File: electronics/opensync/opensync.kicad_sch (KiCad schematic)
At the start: 0 parts

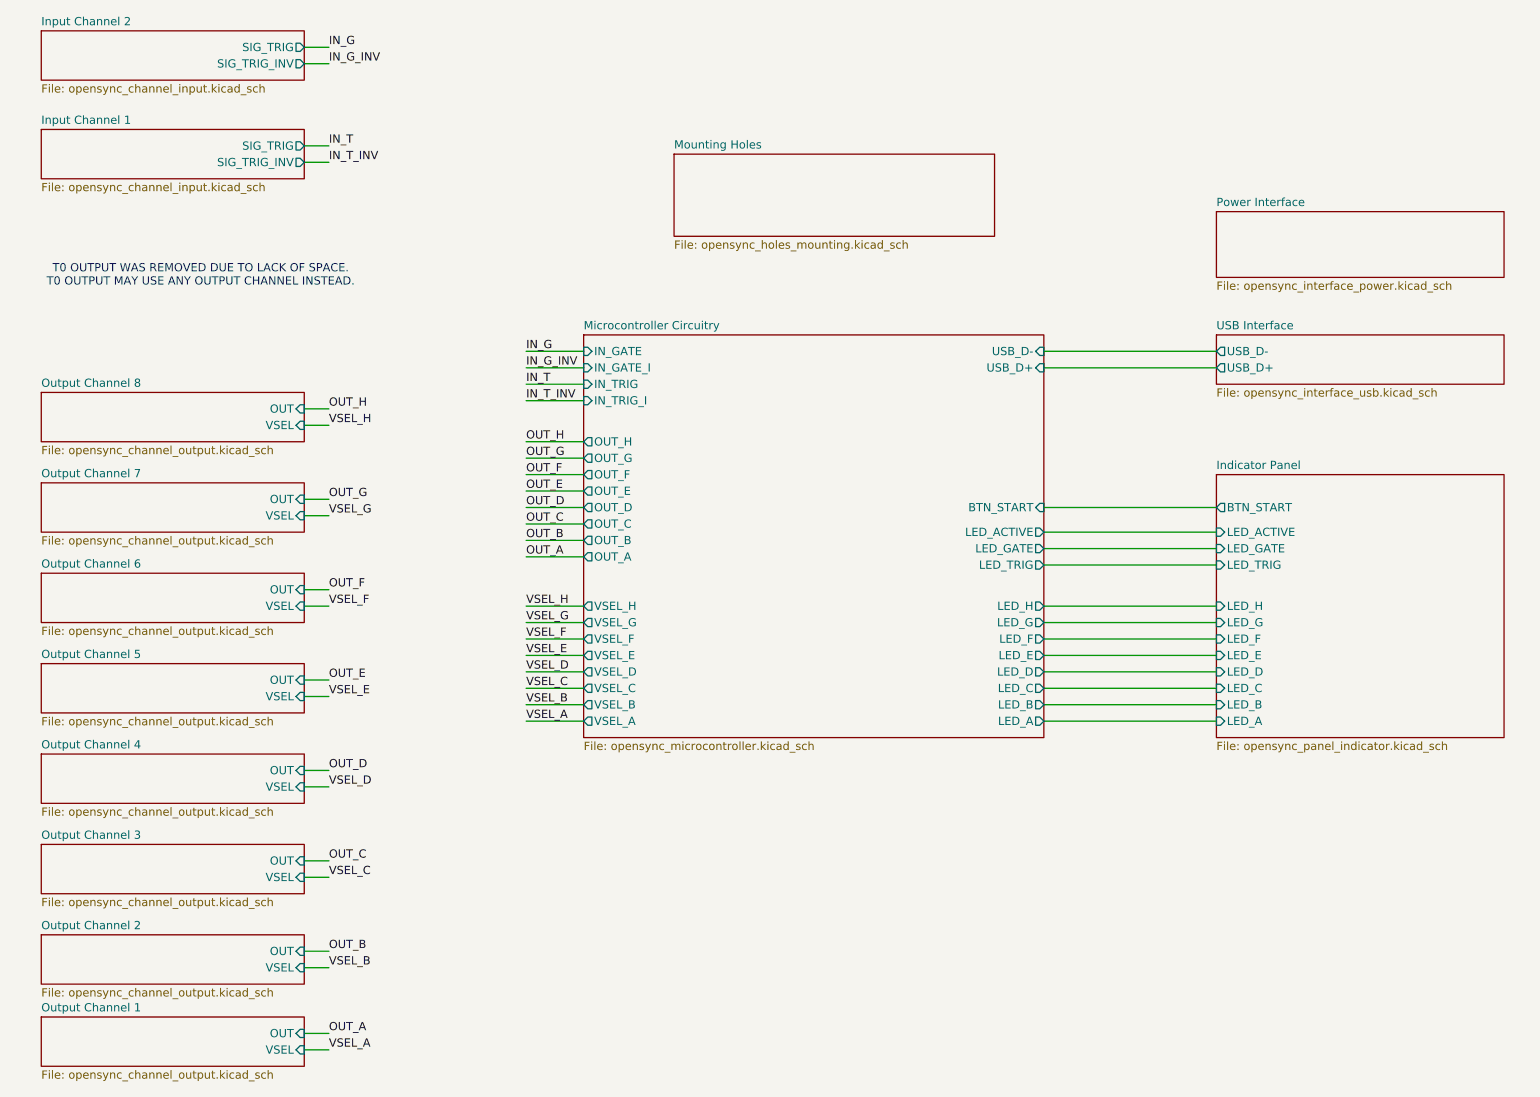
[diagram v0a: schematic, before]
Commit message: Updated new design; getting new PCBs
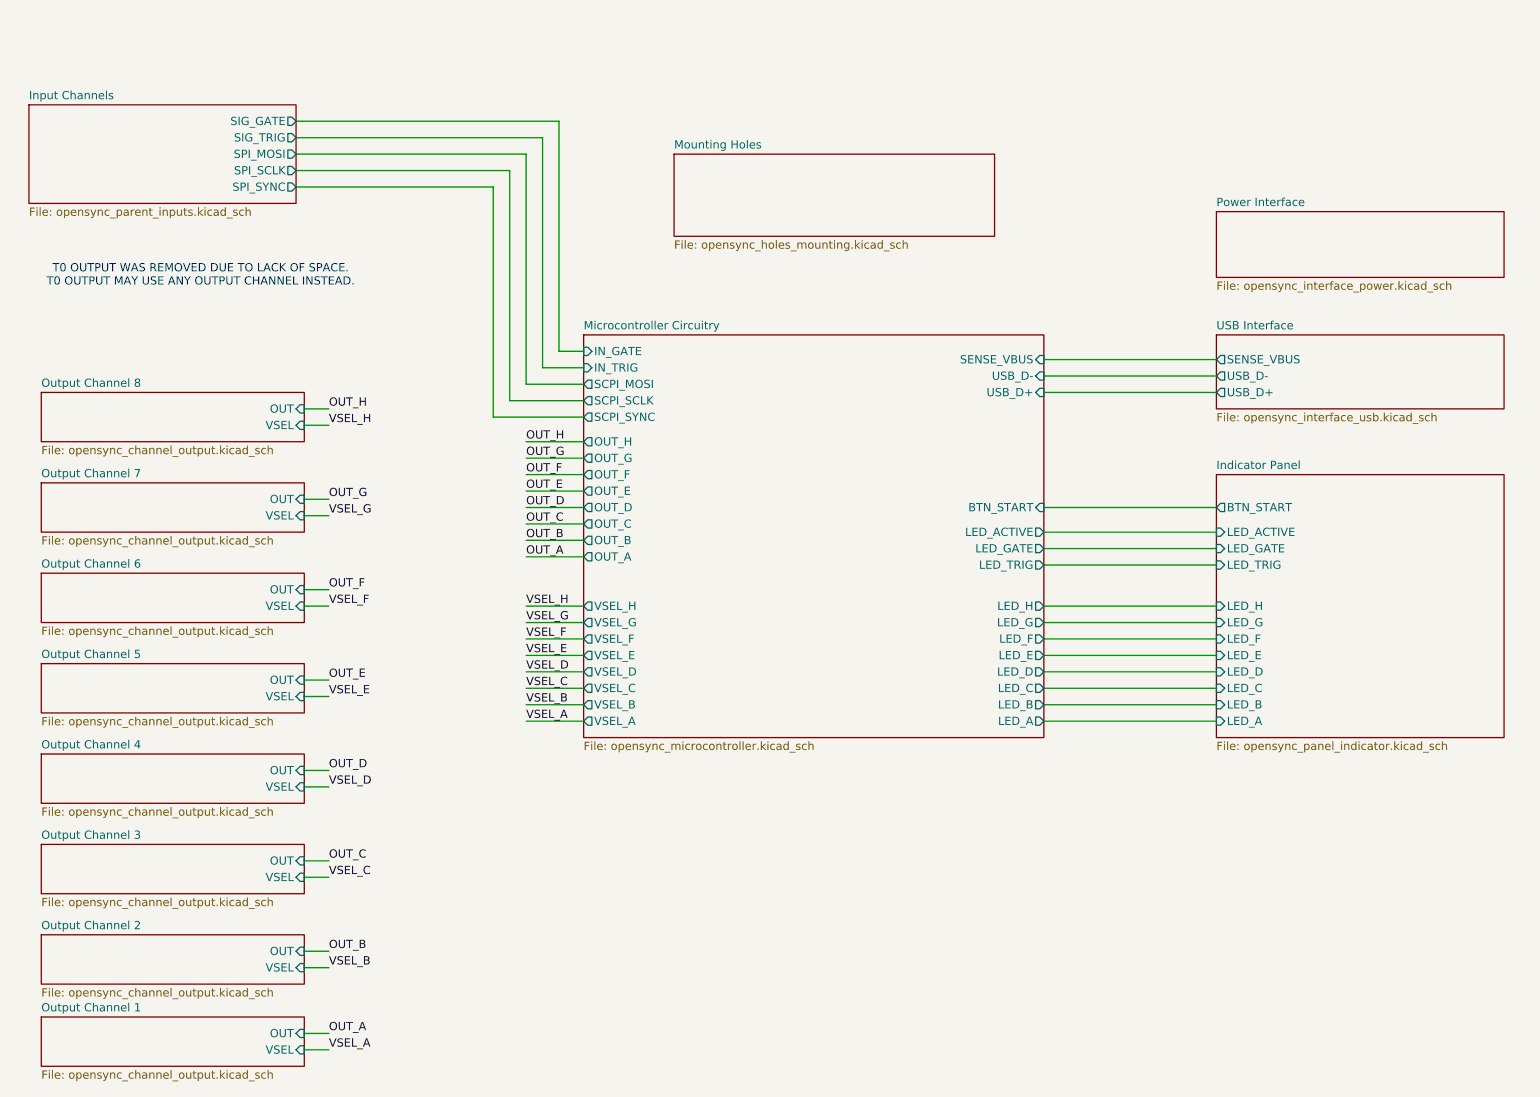
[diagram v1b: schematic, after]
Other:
- removed sheet Input Channel 1
- removed sheet Input Channel 2
- added sheet Input Channels (opensync_parent_inputs.kicad_sch)
- sheet Microcontroller Circuitry ports: added SCPI_MOSI, SCPI_SCLK, SCPI_SYNC, SENSE_VBUS; removed IN_GATE_I, IN_TRIG_I
- sheet USB Interface ports: added SENSE_VBUS; removed none
